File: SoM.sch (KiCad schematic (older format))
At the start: 19 parts, among them J7 MC-HVT1-S04-G, U10 SA800U-WF

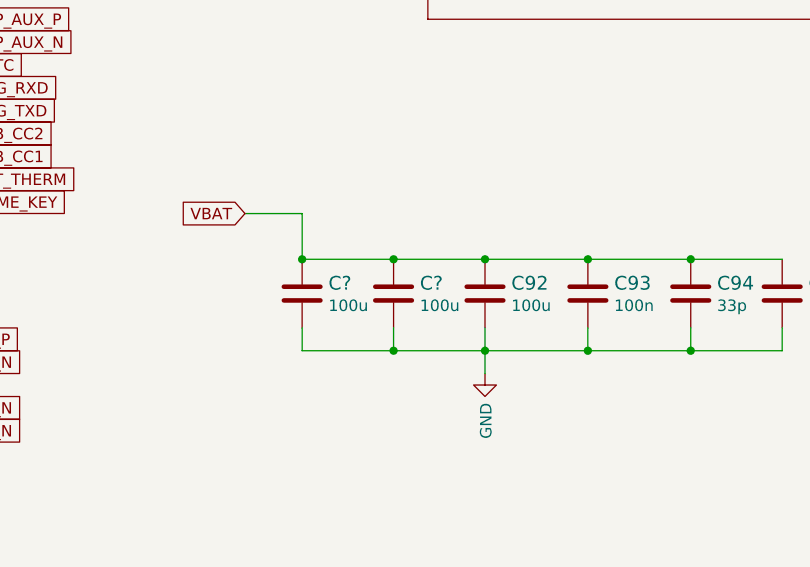
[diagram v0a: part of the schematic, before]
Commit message: annotations
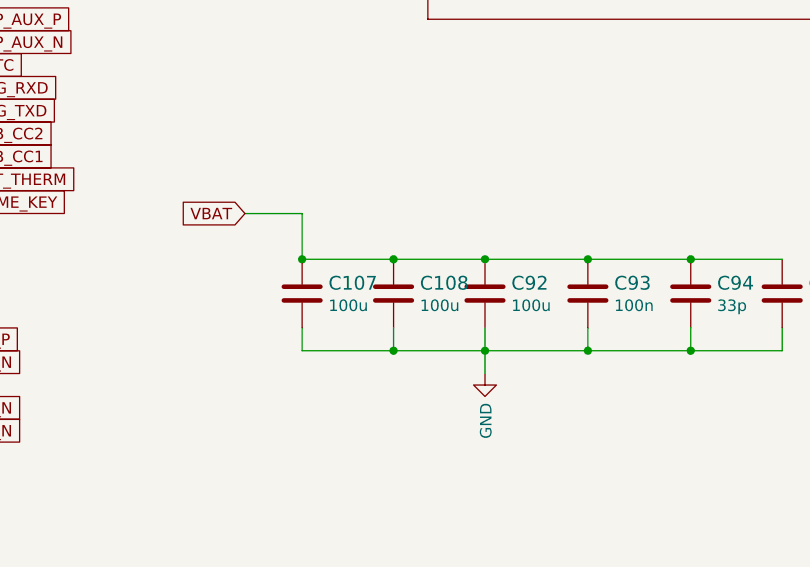
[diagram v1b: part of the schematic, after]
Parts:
- gave numbers to parts that had none: 2
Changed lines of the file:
@@
 VBAT
 $Comp
-L sa800u-baseboard-hw:C_100u_0805 C?
+L sa800u-baseboard-hw:C_100u_0805 C108
 U 1 1 620055D3
 P 12150 9100
-F 0 "C?" H 12265 9145 60  0000 L CNN
+F 0 "C108" H 12265 9145 60  0000 L CNN
 F 1 "C_100u_0805" H 12150 8950 60  0001 C CNN
 F 2 "sa800u-baseboard-hw-footprints:0805-cap" H 12350 9300 60  0001 L CNN
@@
 $EndComp
 $Comp
-L sa800u-baseboard-hw:C_100u_0805 C?
+L sa800u-baseboard-hw:C_100u_0805 C107
 U 1 1 62006DC2
 P 11750 9100
-F 0 "C?" H 11865 9145 60  0000 L CNN
+F 0 "C107" H 11865 9145 60  0000 L CNN
 F 1 "C_100u_0805" H 11750 8950 60  0001 C CNN
 F 2 "sa800u-baseboard-hw-footprints:0805-cap" H 11950 9300 60  0001 L CNN
